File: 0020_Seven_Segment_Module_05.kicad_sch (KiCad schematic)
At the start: 7 parts, among them IC1 74HCT125PW,118, U1 CA56-12CGKWA, U2 MAX7219

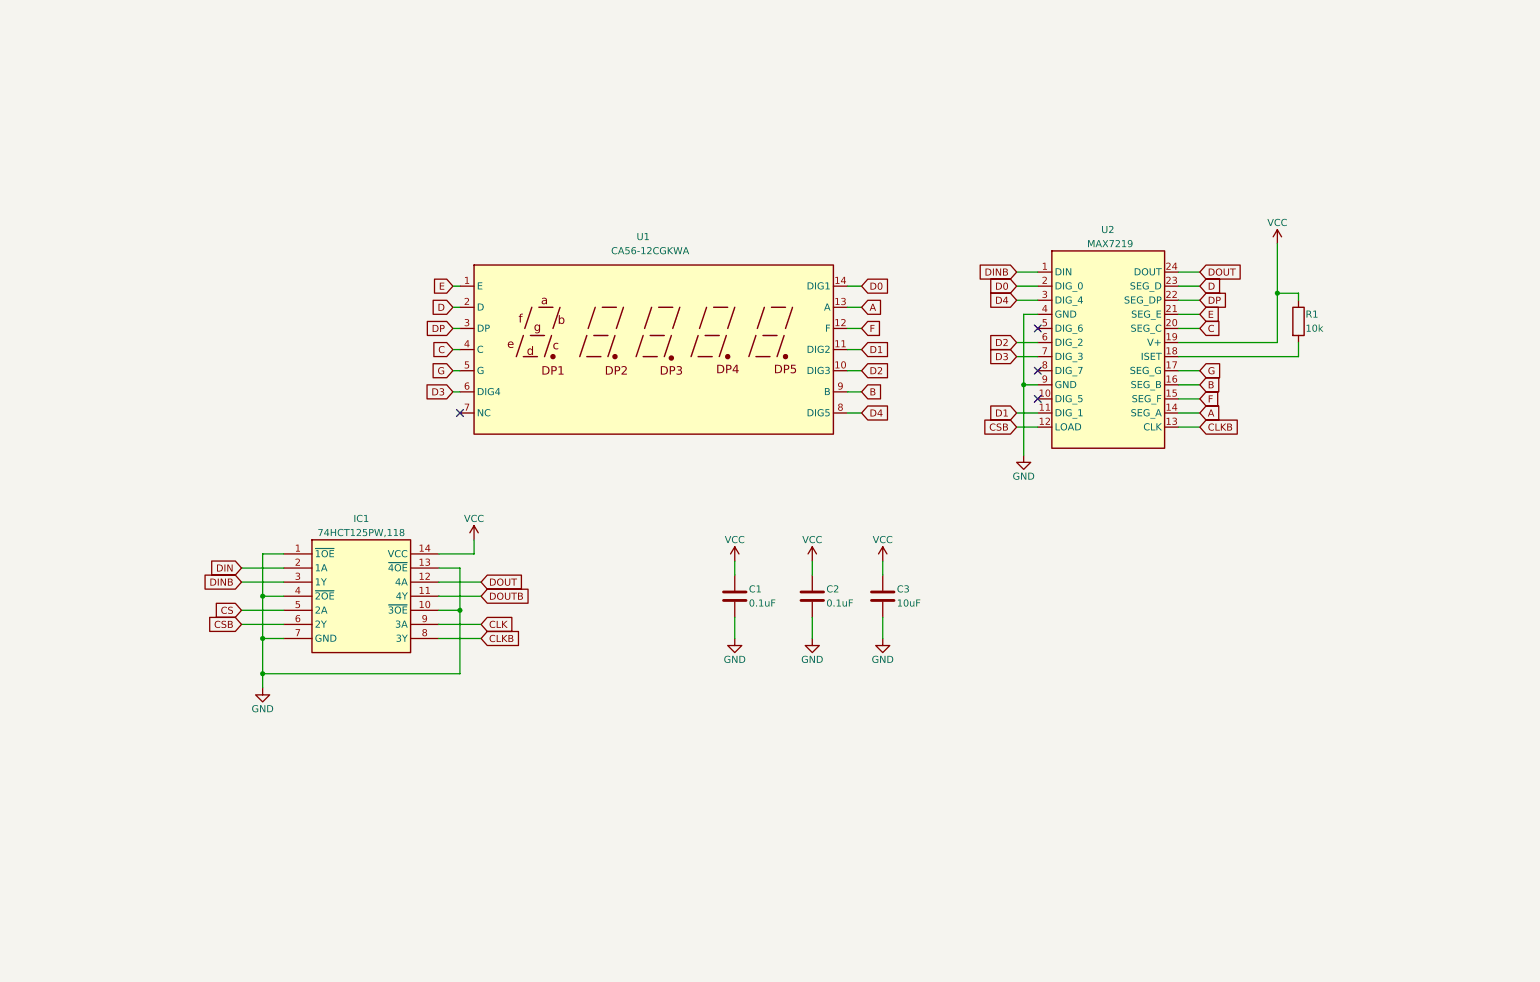
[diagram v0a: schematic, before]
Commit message: Add files via upload
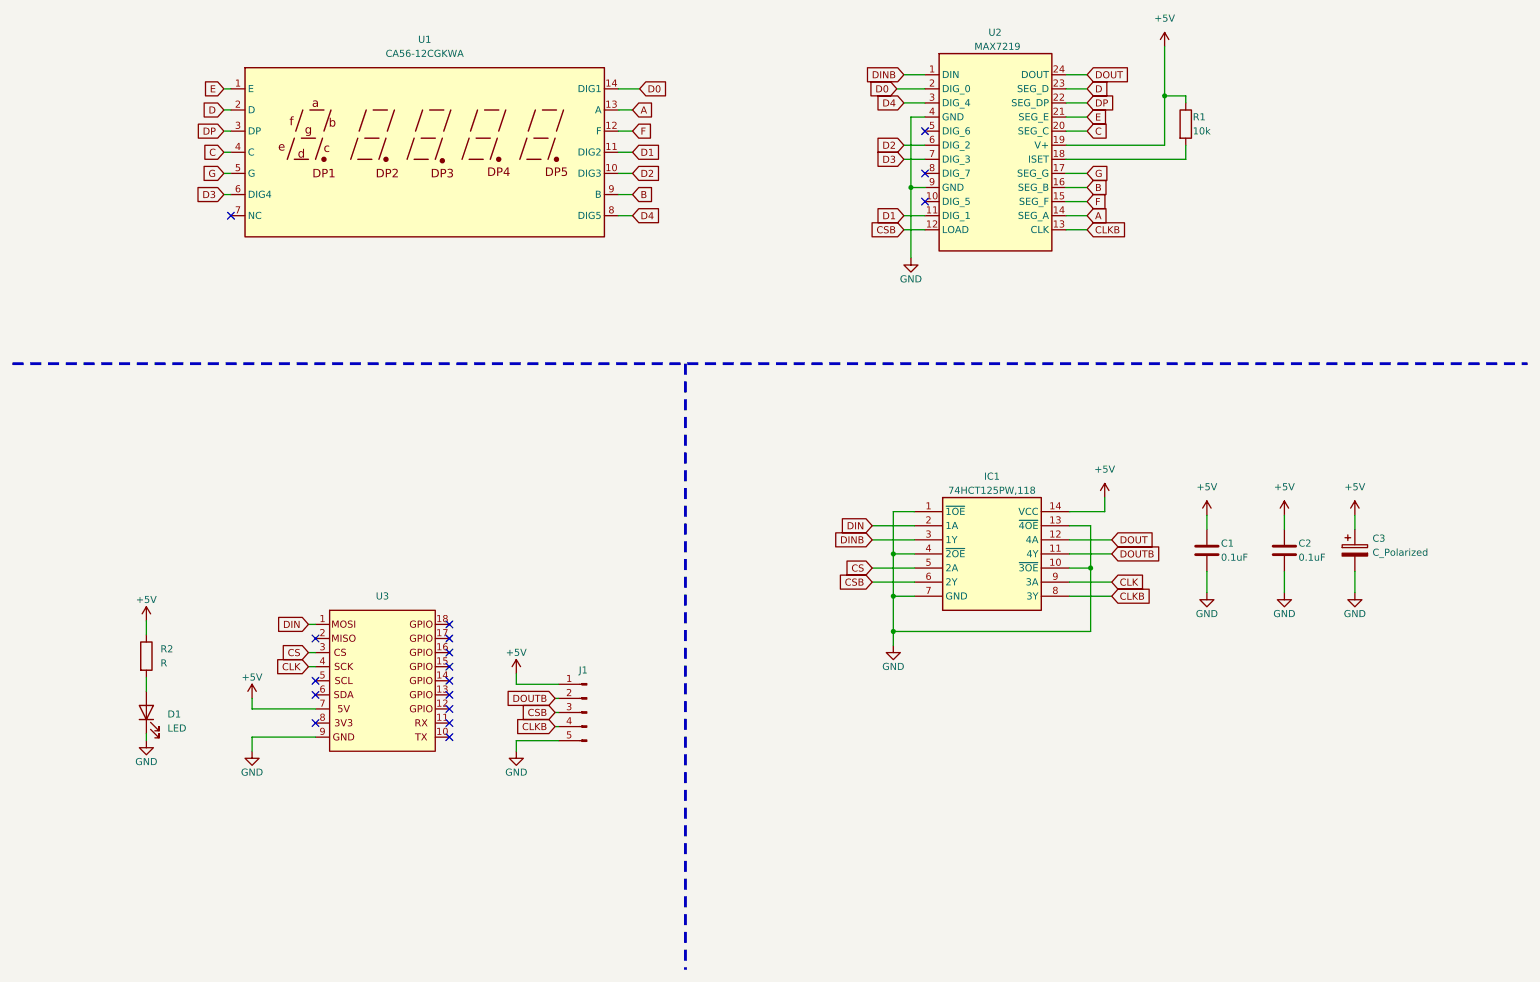
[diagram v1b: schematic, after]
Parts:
- removed C3: 10uF, symbol Device:C
- added C3: C_Polarized, Capacitor_Tantalum_SMD:CP_EIA-3216-10_Kemet-I, symbol Device:C_Polarized
- added D1: LED, LED_SMD:LED_0603_1608Metric, symbol Device:LED
- added J1: Conn_01x05_Pin, Connector_PinHeader_2.54mm:PinHeader_1x05_P2.54mm_Vertical, symbol Connector:Conn_01x05_Pin
- added R2: R, Resistor_SMD:R_0603_1608Metric, symbol Device:R
- added U3: ~, Moduler_:pin_header_5-3, symbol moduler_pin:air
- C1, C2: footprint (none) -> Capacitor_SMD:C_0805_2012Metric
- IC1: footprint SOP65P640X110-14N -> 74LVC125APW:SOP65P640X110-14N
- R1: footprint (none) -> Resistor_SMD:R_0805_2012Metric
- U1: footprint (none) -> meminle:CA56-12CGKWA
- U2: footprint (none) -> Package_SO:SOIC-24W_7.5x15.4mm_P1.27mm
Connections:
- net CLK: now also U3.4
- net CLKB: now also J1.4 (Pin_4)
- net CS: now also U3.3
- net CSB: now also J1.3 (Pin_3)
- net DIN: now also U3.1
- net DOUTB: now also J1.2 (Pin_2)
- net GND: now also C3.2, D1.1 (K), J1.5 (Pin_5), U3.9
- net VCC renamed +5V
- net +5V: now also C3.1, J1.1 (Pin_1), R2.1, U3.7
- new net: D1.2 (A), R2.2
- no-connect marks 4 -> 17
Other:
- moved on the sheet: C1, C2, IC1, R1, U1, U2
